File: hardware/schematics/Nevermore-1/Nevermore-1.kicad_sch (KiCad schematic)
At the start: 2 parts, among them U1 XIAO-ESP32-S3-SMD, U2 MPU-6050

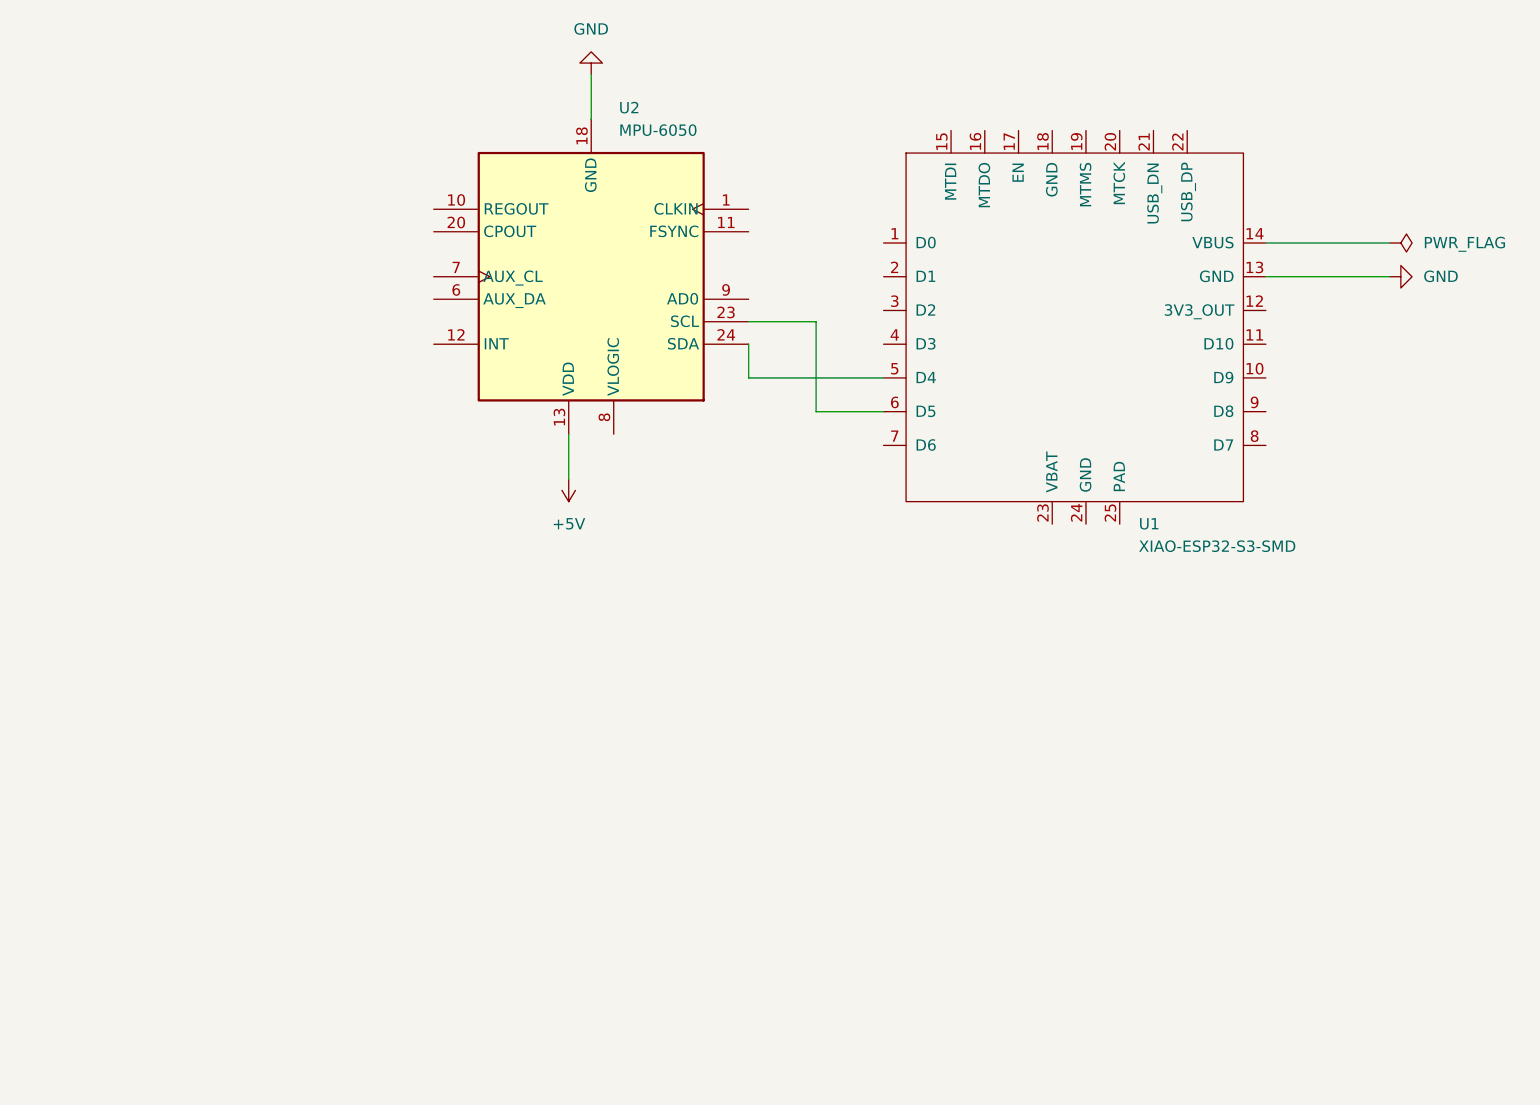
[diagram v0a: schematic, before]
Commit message: Remove lock files for Nevermore-1 schematics to clean up project directory
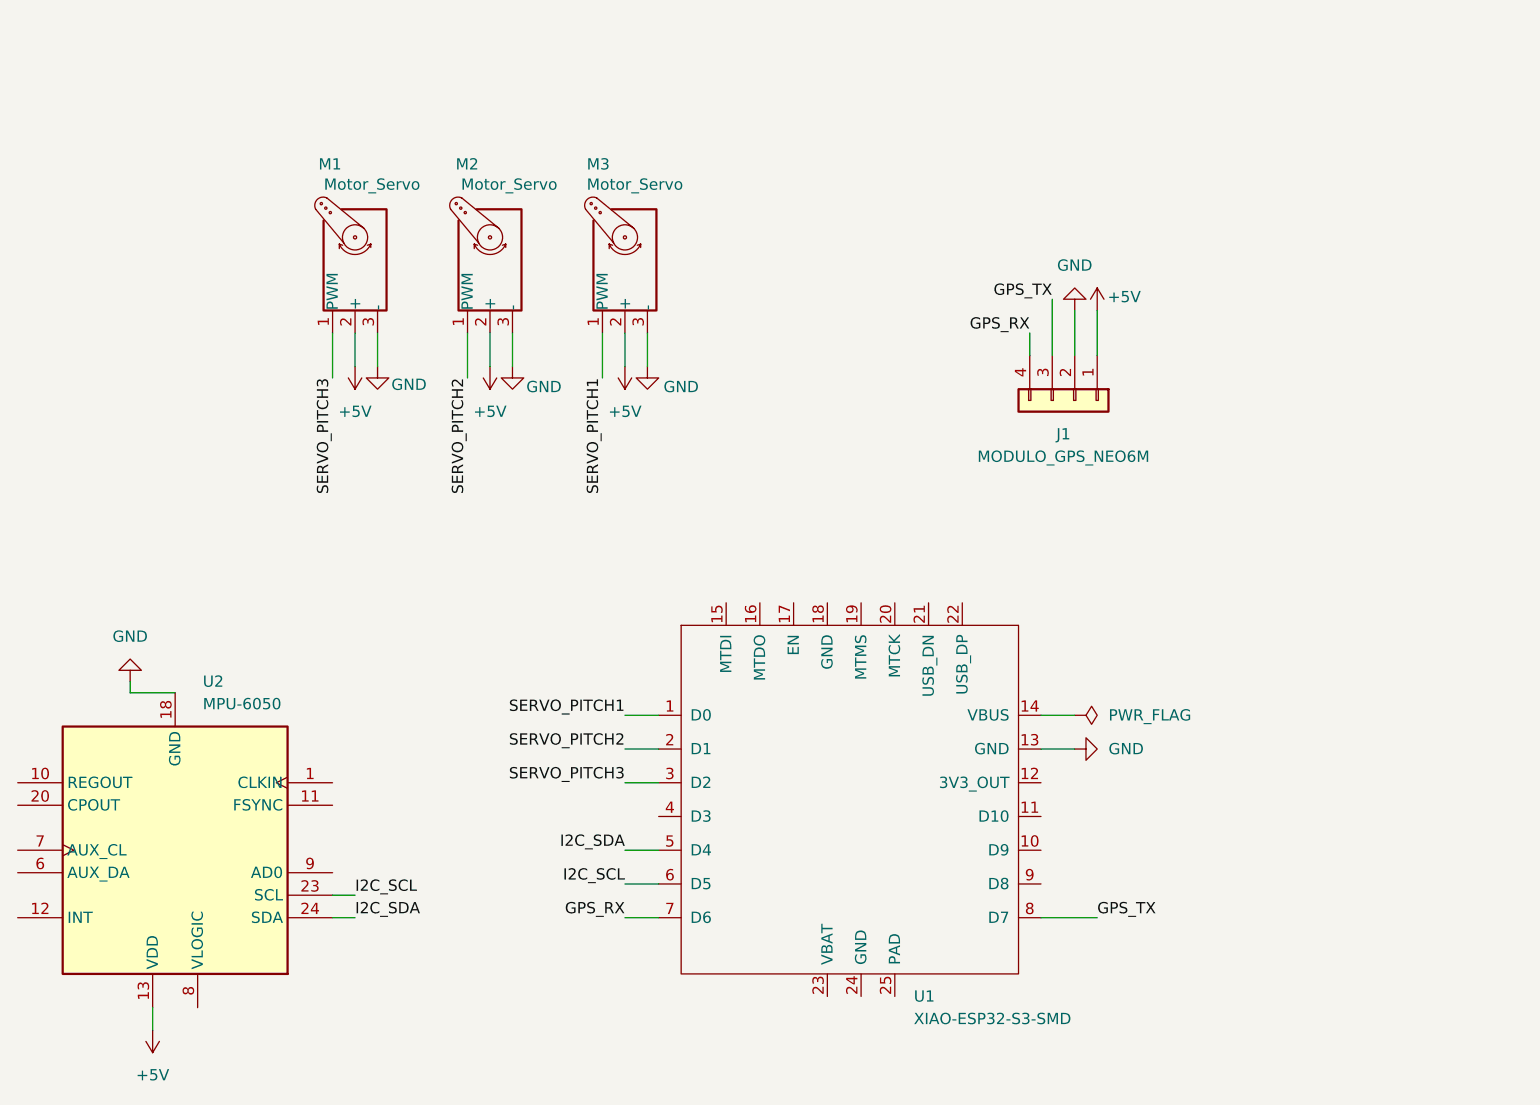
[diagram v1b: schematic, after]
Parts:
- added J1: MODULO_GPS_NEO6M, symbol Connector_Generic:Conn_01x04
- added M1, M2, M3: Motor_Servo, symbol Motor:Motor_Servo
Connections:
- net +5V: now also J1.1 (Pin_1), M1.2 (+), M2.2 (+), M3.2 (+)
- net GND: now also J1.2 (Pin_2), M1.3 (-), M2.3 (-), M3.3 (-)
- net I2C_SCL: now reaches U1.6 (D5), U2.23 (SCL)
- net I2C_SDA: now reaches U1.5 (D4), U2.24 (SDA)
- net SERVO_PITCH1: now reaches U1.1 (D0)
- net SERVO_PITCH1: now also M3.1 (PWM)
- net SERVO_PITCH2: now reaches U1.2 (D1)
- net SERVO_PITCH2: now also M2.1 (PWM)
- net SERVO_PITCH3: now reaches U1.3 (D2)
- net SERVO_PITCH3: now also M1.1 (PWM)
- net GPS_RX: now reaches U1.7 (D6)
- net GPS_RX: now also J1.4 (Pin_4)
- net GPS_TX: now reaches U1.8 (D7)
- net GPS_TX: now also J1.3 (Pin_3)
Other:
- moved on the sheet: U1, U2
